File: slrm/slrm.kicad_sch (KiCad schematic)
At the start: 16 parts, among them J1 Conn_01x08_Male, J8 Conn_01x08_Male

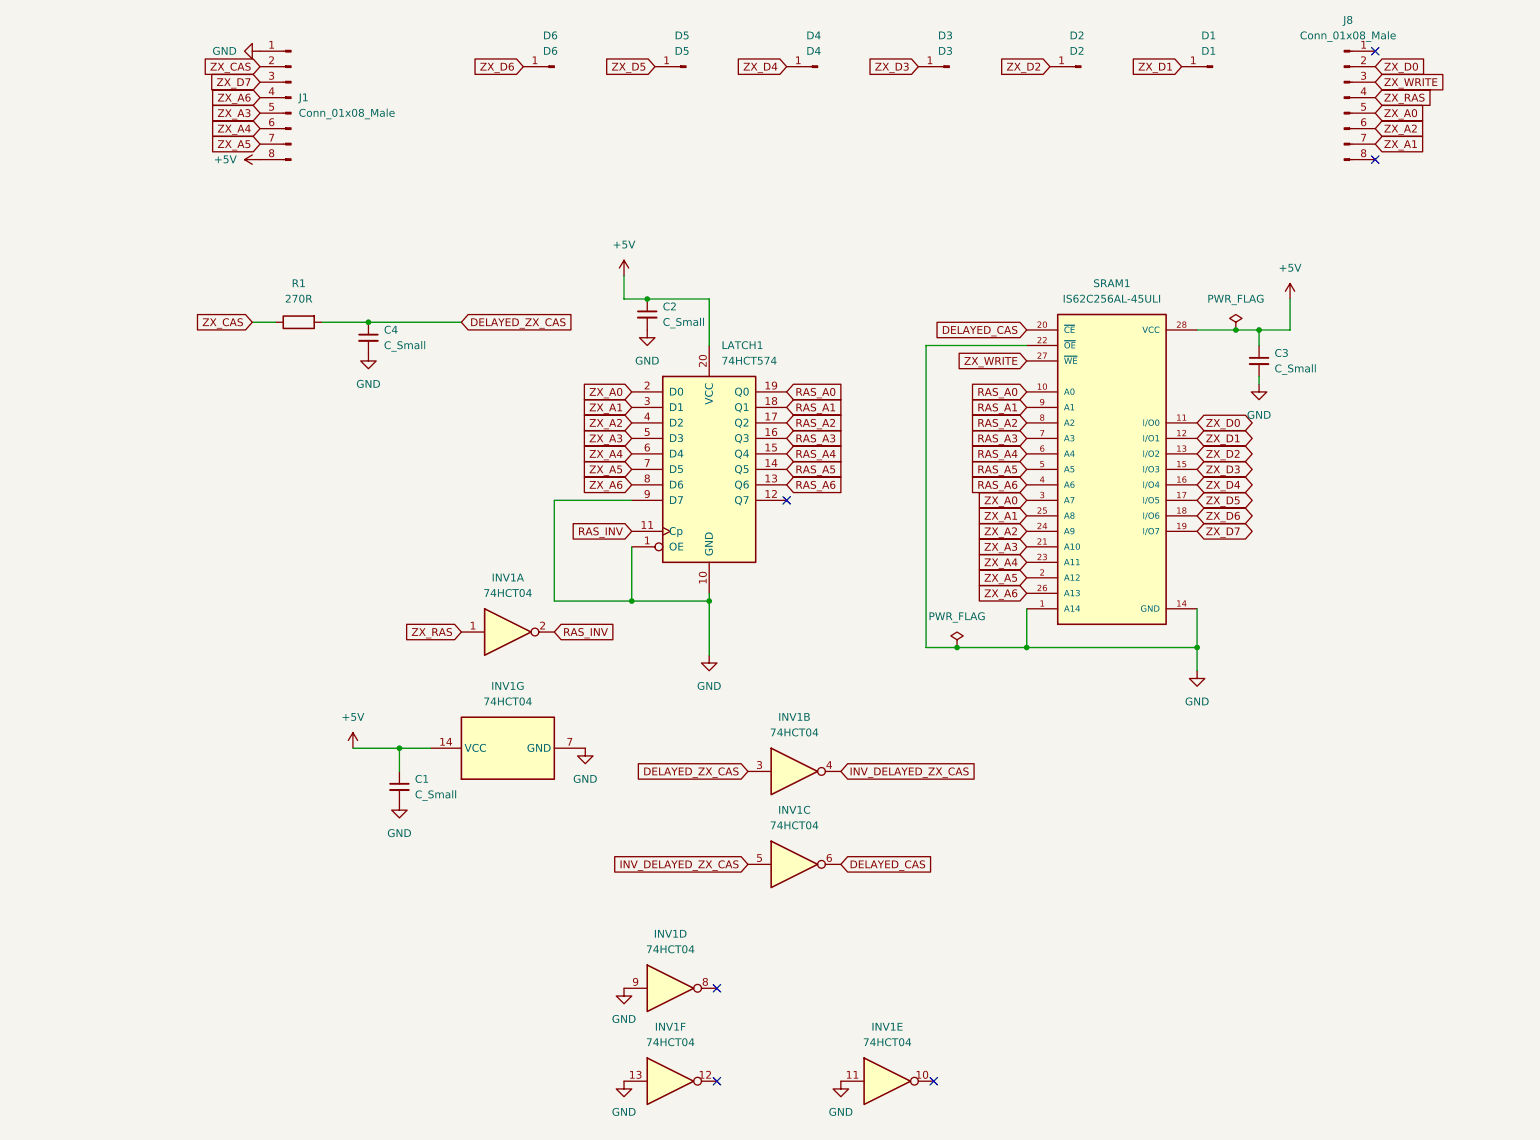
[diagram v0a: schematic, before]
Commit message: version 1.2 gerbers created
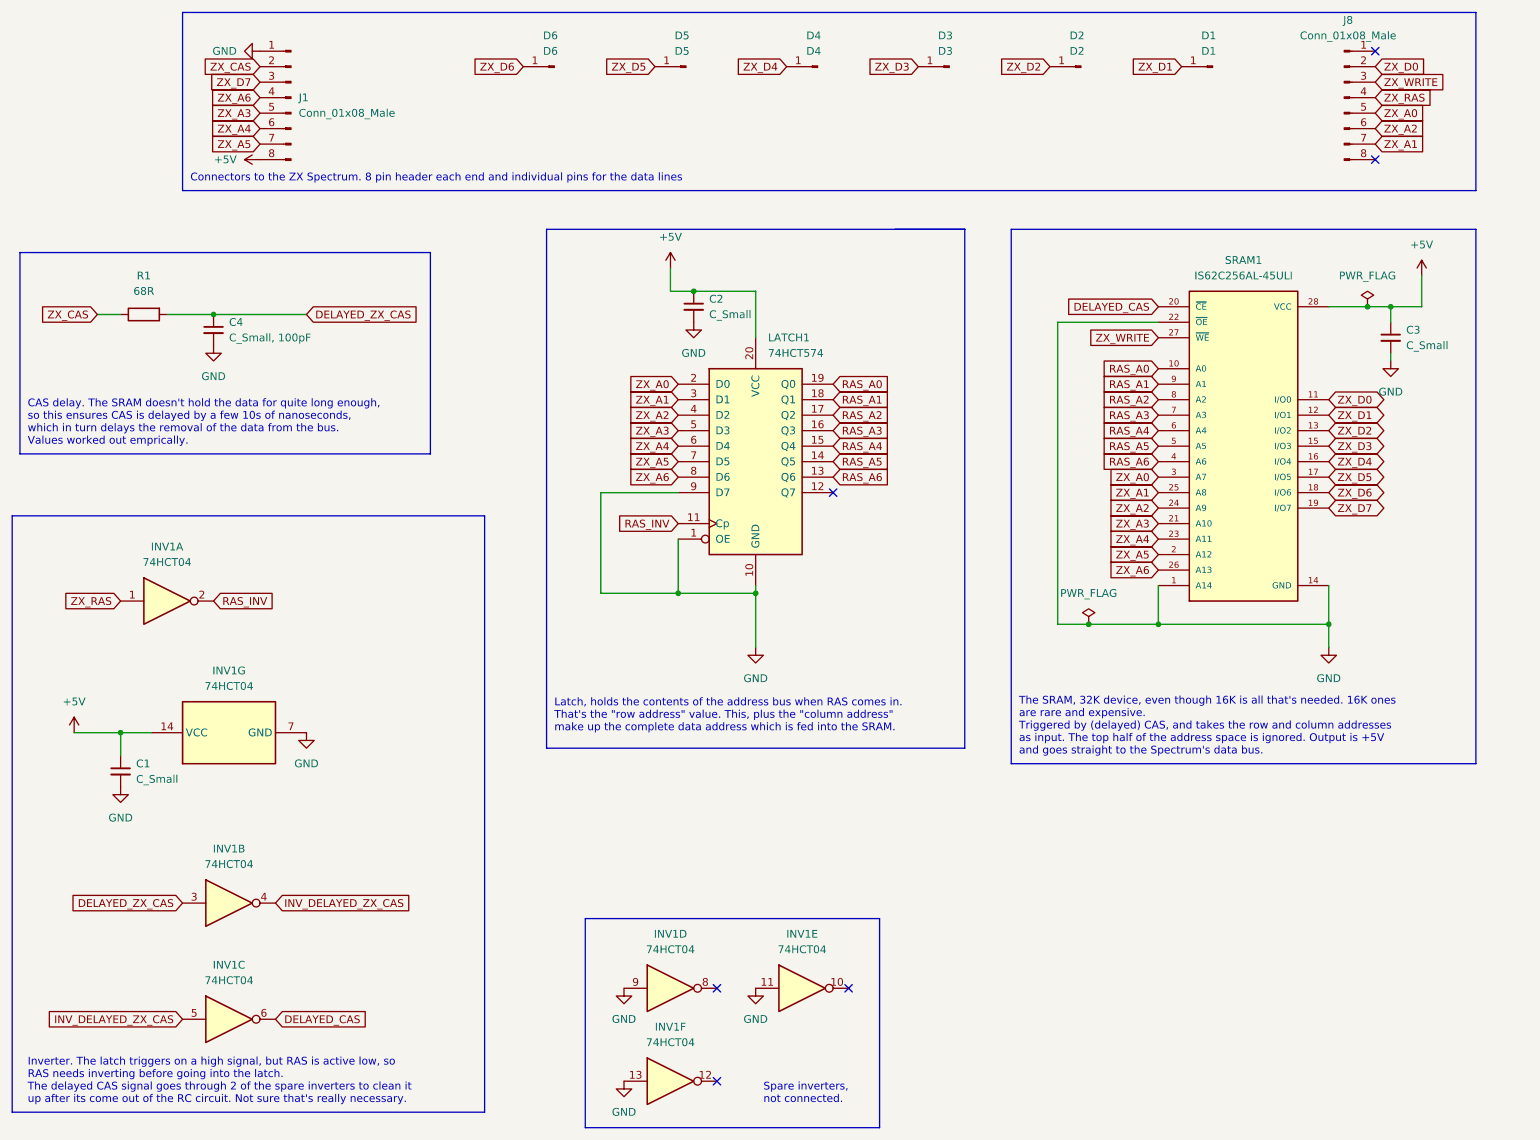
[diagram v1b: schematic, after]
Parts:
- C4: value C_Small -> C_Small, 100pF
- R1: value 270R -> 68R
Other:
- note added: "CAS delay. The SRAM doesn't hold the data for quite long enough, so this ensures CAS is delayed by a few 10s of nanoseconds, which in turn delays the removal of the data from the bus. Values worked out emprically."
- note added: "Connectors to the ZX Spectrum. 8 pin header each end and individual pins for the data lines"
- note added: "Inverter. The latch triggers on a high signal, but RAS is active low, so RAS needs inverting before going into the latch. The delayed CAS signal goes through 2 of the spare inverters to clean it up after its come out of the RC circuit. Not sure that's really necessary."
- note added: "Latch, holds the contents of the address bus when RAS comes in. That's the "row address" value. This, plus the "column address" make up the complete data address which is fed into the SRAM."
- note added: "Spare inverters, not connected."
- note added: "The SRAM, 32K device, even though 16K is all that's needed. 16K ones are rare and expensive. Triggered by (delayed) CAS, and takes the row and column addresses as input. The top half of the address space is ignored. Output is +5V and goes straight to the Spectrum's data bus."
- title: (none) -> ZX Spectrum Lower RAM Module
- moved on the sheet: C1, C2, C3, C4, INV1A, INV1B, INV1C, INV1E, INV1G, LATCH1, R1, SRAM1
